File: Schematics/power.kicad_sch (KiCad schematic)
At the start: 8 parts, among them U5 AMS1117-3.3

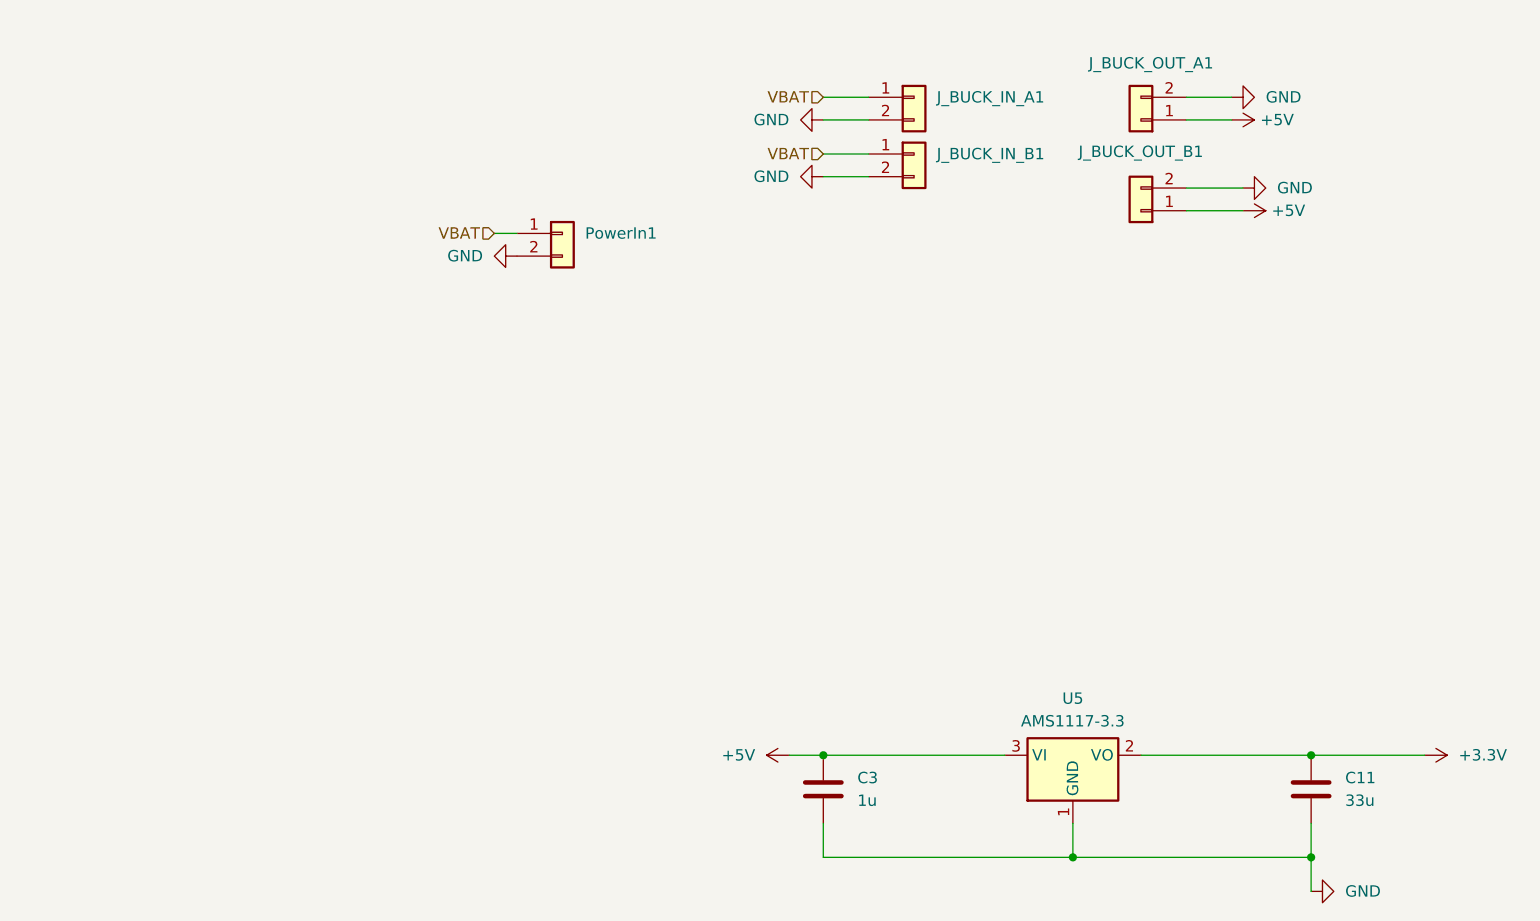
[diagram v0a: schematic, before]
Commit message: Cleaned up schematic added ocilator added jtag 10 pin begining routing again
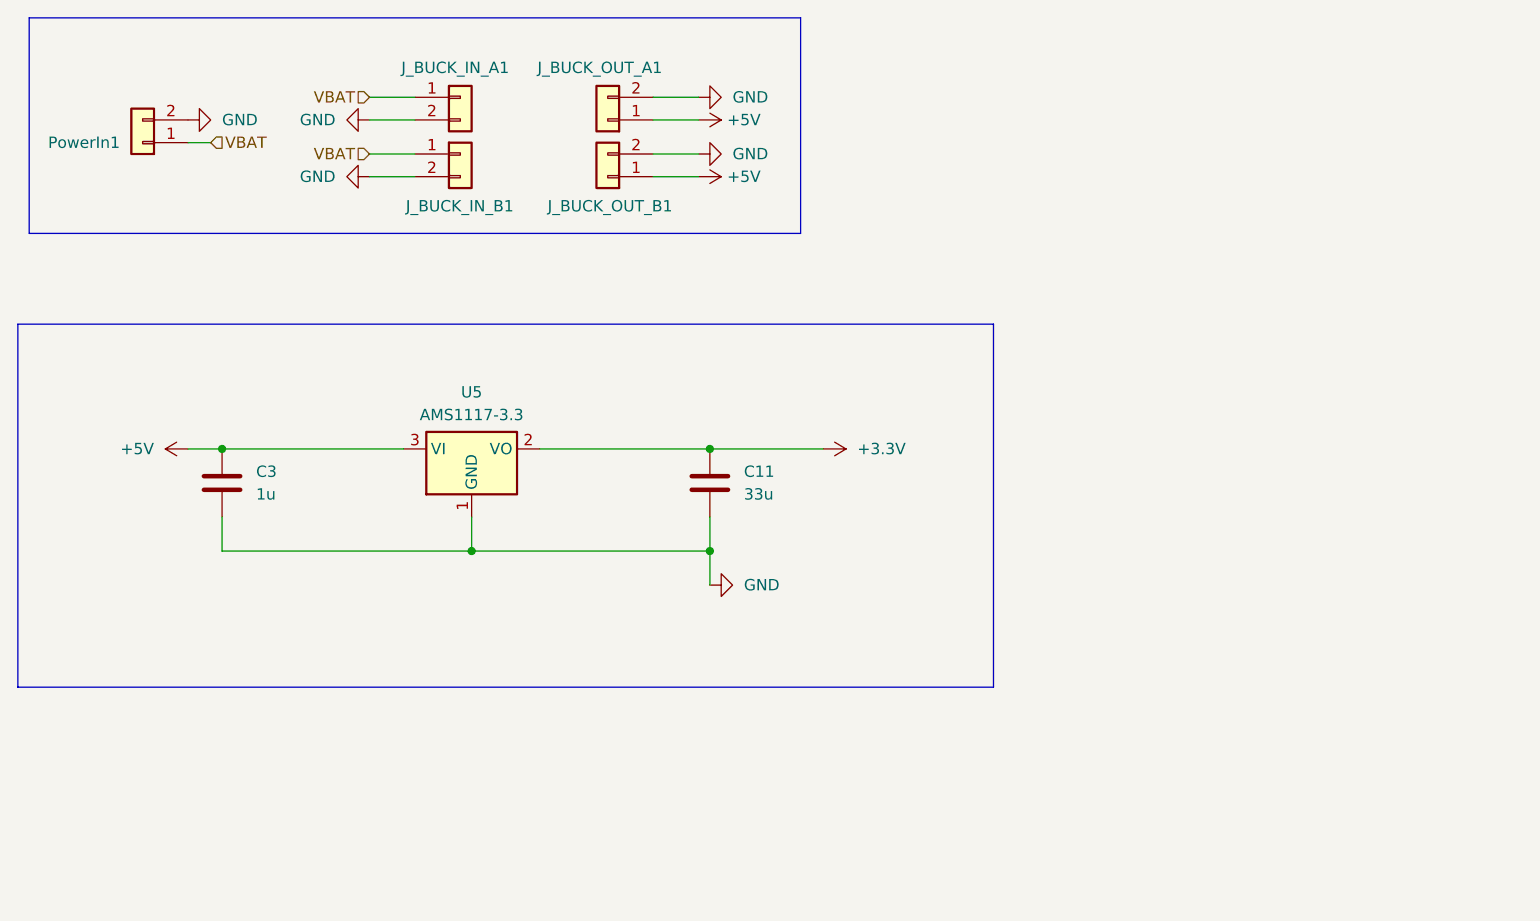
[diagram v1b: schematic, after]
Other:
- moved on the sheet: C11, C3, J_BUCK_IN_A1, J_BUCK_IN_B1, J_BUCK_OUT_A1, J_BUCK_OUT_B1, PowerIn1, U5
